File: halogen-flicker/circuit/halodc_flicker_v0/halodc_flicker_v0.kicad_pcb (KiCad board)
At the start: 2 copper layers, 86.1 x 45.6 mm, 21 parts, among them J1 ASP, J2 BATT_LAMP, J4 CHARGER, Q1 IRF540N, SW1 SW_DIP_x02, SW2 SW_Push, U1 ATtiny13A-S, U2 PC817, U3 AMS1117-5.0

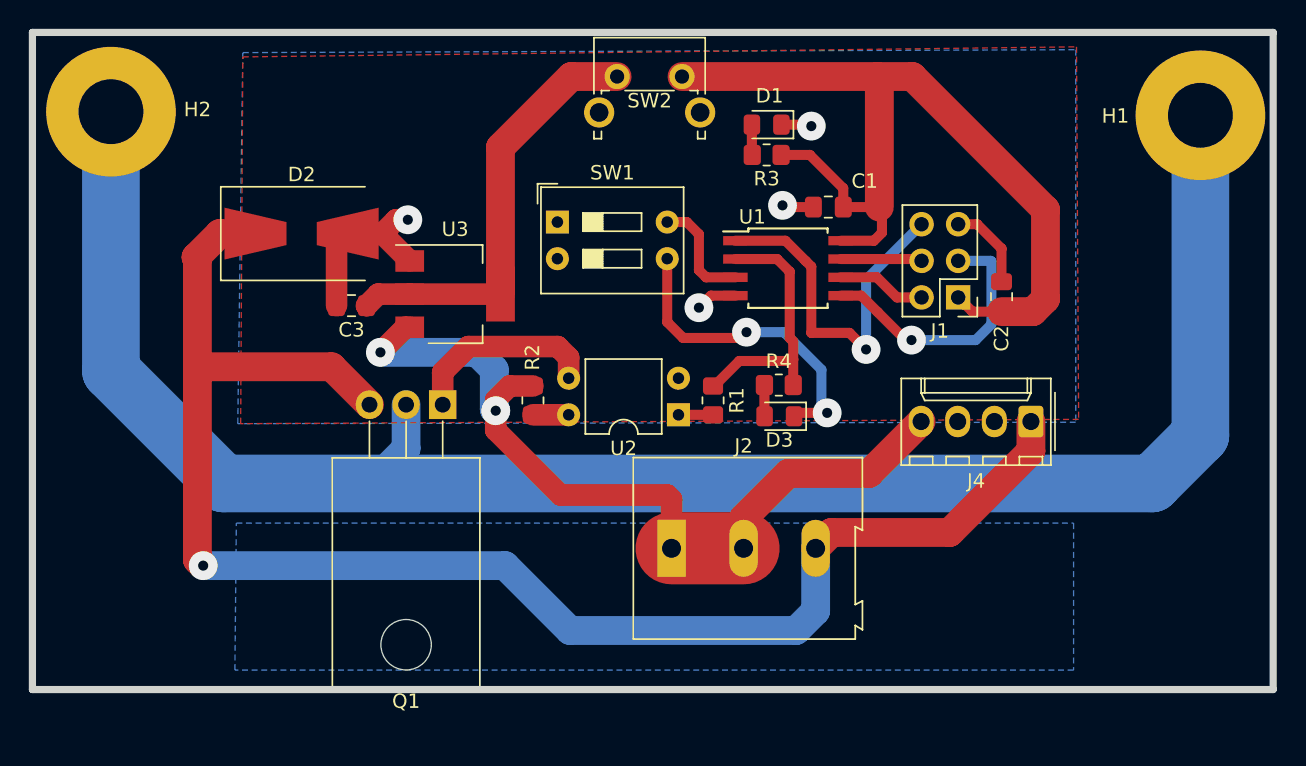
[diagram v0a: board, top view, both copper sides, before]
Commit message: Update PCB FLicker Halogen
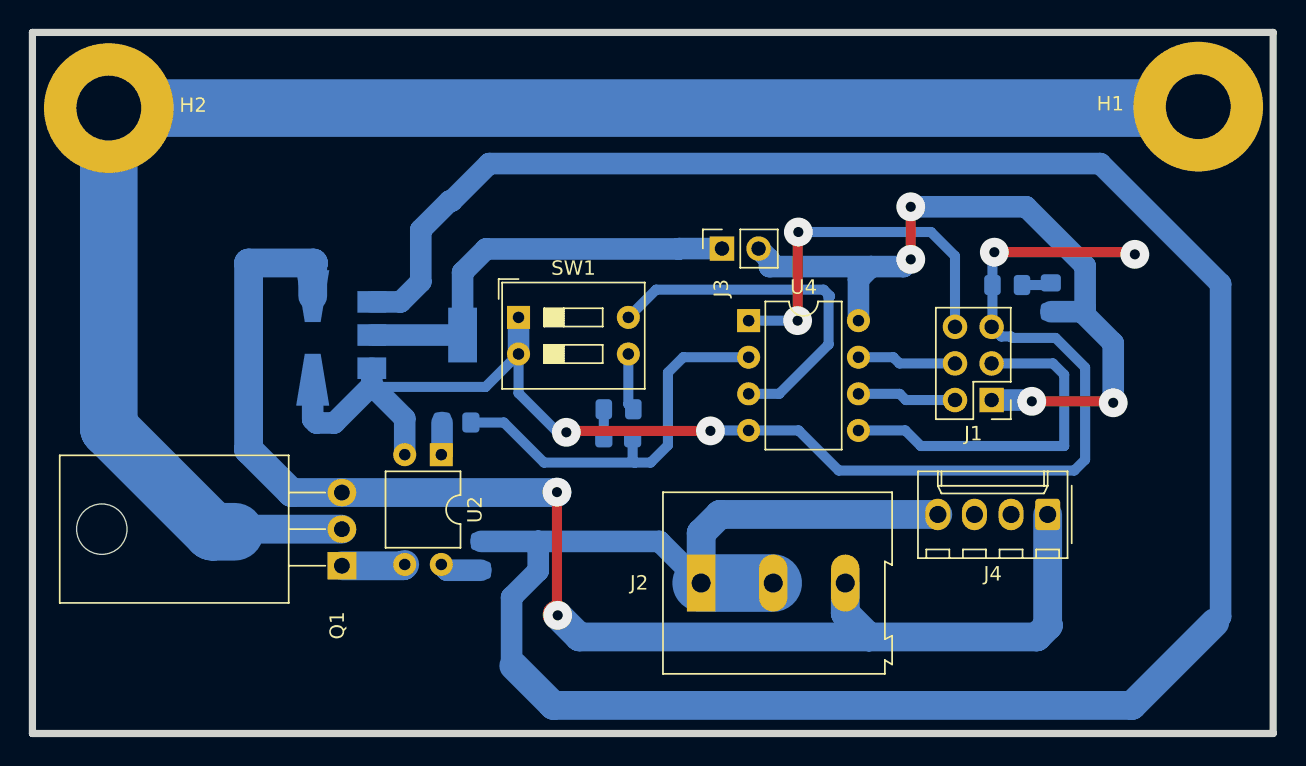
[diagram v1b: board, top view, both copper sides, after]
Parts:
- removed C1, C2, C3: 100nF, Capacitor_SMD:C_0805_2012Metric_Pad1.18x1.45mm_HandSolder
- removed SW2: SW_Push, Button_Switch_THT:SW_Tactile_SPST_Angled_PTS645Vx31-2LFS
- removed U1: ATtiny13A-S, Package_SO:SOIC-8W_5.3x5.3mm_P1.27mm
- added J3: SW_ON, Connector_PinSocket_2.54mm:PinSocket_1x02_P2.54mm_Vertical, F.Cu at (121.2, 54.5)
- added U4: ATtiny13A-P, Package_DIP:DIP-8_W7.62mm, F.Cu at (123.0, 59.5)
- D1, D3, R1, R2, R3, R4, U3: moved to B.Cu
- D2: footprint Diode_SMD:D_SMB-SMC_Universal_Handsoldering -> Diode_SMD:D_SMA-SMB_Universal_Handsoldering; moved to B.Cu
- moved R3 22.1 mm to (144.0, 57.8), turned to 90 degrees
- moved D1 20.1 mm to (140.9, 57.0), turned to 0 degrees
- moved R1 17.9 mm to (102.7, 66.5), turned to 180 degrees
- moved U2 16.7 mm to (101.7, 68.8), turned to -90 degrees
- moved Q1 13.2 mm to (94.8, 76.5), turned to 90 degrees
- moved R4 11.7 mm to (114.0, 67.5)
- moved R2 11.4 mm to (104.4, 75.8)
- moved D3 11.2 mm to (114.0, 65.6)
- moved J1 7.49 mm to (139.9, 65.0)
- moved D2 7.28 mm to (92.8, 60.6), turned to -90 degrees
- moved SW1 7.14 mm to (107.0, 59.2)
- moved J4 6.55 mm to (143.8, 72.9)
- moved U3 3.87 mm to (100.0, 60.5)
- moved J2 3.17 mm to (119.7, 77.7)
- moved H1 0.62 mm to (154.2, 44.6)
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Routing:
- net +12V: track 58.9 -> 195.6 mm, vias 2 -> 0
- net GND: track 25.8 -> 102.5 mm
- net Net-(D3-K): track 22.4 -> 3.98 mm, vias 2 -> 0
- net SEL: track 7.78 -> 25.3 mm
- net +5V: track 65.2 -> 54.7 mm, vias 0 -> 4
- net GNDREF: track 108.5 -> 98.1 mm, vias 1 -> 2
- net CON: track 18.4 -> 28.2 mm
- net Net-(Q1-G): track 13.5 -> 4.40 mm
- net GNDPWR: track 125.6 -> 117.1 mm
- net MOSI: track 18.9 -> 25.0 mm, vias 1 -> 0
- net SCK: track 5.67 -> 6.88 mm
- net NRST: track 25.2 -> 26.0 mm, vias 1 -> 2
- net MISO: track 6.20 -> 6.88 mm
- net Net-(J3-Pin_1): track 29.9 -> 29.3 mm
- added copper zone on B.Cu, net (none)
- removed copper zone on F.Cu, net (none)
- removed copper zone on B.Cu, net GND
- removed copper zone on B.Cu, net GNDREF
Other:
- board size 86.1 x 45.6 mm -> 86.1 x 48.6 mm

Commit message: Update PCB FLicker
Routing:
- added copper zone on F.Cu, net (none)
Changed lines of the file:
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@@
     (fp_line (start 8.89 2.88) (end 8.89 -2.92)
       (stroke (width 0.1) (type solid)) (layer "F.Fab"))
-    (pad "1" thru_hole roundrect (at 0 0 180) (size 1.74 2.19) (drill 1.19) (layers "*.Cu" "*.Mask") (roundrect_rratio 0.143678)
+    (pad "1" thru_hole roundrect (at 0 0 180) (size 1.74 2.19) (drill 1.19) (layers "*.Cu" "*.Mask") (roundrect_rratio 0.1436781609)
       (net 5 "GNDREF") (pinfunction "Pin_1") (pintype "passive"))
     (pad "2" thru_hole oval (at 2.54 0 180) (size 1.74 2.19) (drill 1.19) (layers "*.Cu" "*.Mask")
@@
     (fp_line (start 1 0.625) (end 1 -0.625)
       (stroke (width 0.1) (type solid)) (layer "B.Fab"))
-    (pad "1" smd roundrect (at -1 0 90) (size 1.2 1.4) (layers "B.Cu" "B.Paste" "B.Mask") (roundrect_rratio 0.208333)
+    (pad "1" smd roundrect (at -1 0 90) (size 1.2 1.4) (layers "B.Cu" "B.Paste" "B.Mask") (roundrect_rratio 0.2083333333)
       (net 1 "+5V") (pintype "passive"))
-    (pad "2" smd roundrect (at 1 0 90) (size 1.2 1.4) (layers "B.Cu" "B.Paste" "B.Mask") (roundrect_rratio 0.208333)
+    (pad "2" smd roundrect (at 1 0 90) (size 1.2 1.4) (layers "B.Cu" "B.Paste" "B.Mask") (roundrect_rratio 0.2083333333)
       (net 4 "Net-(D1-A)") (pintype "passive"))
     (model "${KICAD6_3DMODEL_DIR}/Resistor_SMD.3dshapes/R_0805_2012Metric.wrl"
@@
     (fp_line (start 1 0.625) (end 1 -0.625)
       (stroke (width 0.1) (type solid)) (layer "B.Fab"))
-    (pad "1" smd roundrect (at -1 0) (size 1.2 1.4) (layers "B.Cu" "B.Paste" "B.Mask") (roundrect_rratio 0.208333)
+    (pad "1" smd roundrect (at -1 0) (size 1.2 1.4) (layers "B.Cu" "B.Paste" "B.Mask") (roundrect_rratio 0.2083333333)
       (net 7 "Net-(D3-A)") (pintype "passive"))
-    (pad "2" smd roundrect (at 1 0) (size 1.2 1.4) (layers "B.Cu" "B.Paste" "B.Mask") (roundrect_rratio 0.208333)
+    (pad "2" smd roundrect (at 1 0) (size 1.2 1.4) (layers "B.Cu" "B.Paste" "B.Mask") (roundrect_rratio 0.2083333333)
       (net 17 "CON") (pintype "passive"))
     (model "${KICAD6_3DMODEL_DIR}/Resistor_SMD.3dshapes/R_0805_2012Metric.wrl"
@@
     (fp_line (start 1 0.6) (end -0.7 0.6)
       (stroke (width 0.1) (type solid)) (layer "B.Fab"))
-    (pad "1" smd roundrect (at -1.025 0) (size 1.15 1.4) (layers "B.Cu" "B.Paste" "B.Mask") (roundrect_rratio 0.217391)
+    (pad "1" smd roundrect (at -1.025 0) (size 1.15 1.4) (layers "B.Cu" "B.Paste" "B.Mask") (roundrect_rratio 0.2173913043)
       (net 2 "GND") (pinfunction "K") (pintype "passive"))
-    (pad "2" smd roundrect (at 1.025 0) (size 1.15 1.4) (layers "B.Cu" "B.Paste" "B.Mask") (roundrect_rratio 0.217391)
+    (pad "2" smd roundrect (at 1.025 0) (size 1.15 1.4) (layers "B.Cu" "B.Paste" "B.Mask") (roundrect_rratio 0.2173913043)
       (net 4 "Net-(D1-A)") (pinfunction "A") (pintype "passive"))
     (model "${KICAD6_3DMODEL_DIR}/LED_SMD.3dshapes/LED_0805_2012Metric.wrl"
@@
     (fp_line (start 1 0.6) (end -0.7 0.6)
       (stroke (width 0.1) (type solid)) (layer "B.Fab"))
-    (pad "1" smd roundrect (at -1.025 0 180) (size 1.15 1.4) (layers "B.Cu" "B.Paste" "B.Mask") (roundrect_rratio 0.217391)
+    (pad "1" smd roundrect (at -1.025 0 180) (size 1.15 1.4) (layers "B.Cu" "B.Paste" "B.Mask") (roundrect_rratio 0.2173913043)
       (net 6 "Net-(D3-K)") (pinfunction "K") (pintype "passive"))
-    (pad "2" smd roundrect (at 1.025 0 180) (size 1.15 1.4) (layers "B.Cu" "B.Paste" "B.Mask") (roundrect_rratio 0.217391)
+    (pad "2" smd roundrect (at 1.025 0 180) (size 1.15 1.4) (layers "B.Cu" "B.Paste" "B.Mask") (roundrect_rratio 0.2173913043)
       (net 7 "Net-(D3-A)") (pinfunction "A") (pintype "passive"))
     (model "${KICAD6_3DMODEL_DIR}/LED_SMD.3dshapes/LED_0805_2012Metric.wrl"
@@
     (fp_line (start 1 0.625) (end 1 -0.625)
       (stroke (width 0.1) (type solid)) (layer "B.Fab"))
-    (pad "1" smd roundrect (at -1 0 180) (size 1.2 1.4) (layers "B.Cu" "B.Paste" "B.Mask") (roundrect_rratio 0.208333)
+    (pad "1" smd roundrect (at -1 0 180) (size 1.2 1.4) (layers "B.Cu" "B.Paste" "B.Mask") (roundrect_rratio 0.2083333333)
       (net 17 "CON") (pintype "passive"))
-    (pad "2" smd roundrect (at 1 0 180) (size 1.2 1.4) (layers "B.Cu" "B.Paste" "B.Mask") (roundrect_rratio 0.208333)
+    (pad "2" smd roundrect (at 1 0 180) (size 1.2 1.4) (layers "B.Cu" "B.Paste" "B.Mask") (roundrect_rratio 0.2083333333)
       (net 18 "Net-(R1-Pad2)") (pintype "passive"))
     (model "${KICAD6_3DMODEL_DIR}/Resistor_SMD.3dshapes/R_0805_2012Metric.wrl"
@@
     (fp_line (start 1 0.625) (end 1 -0.625)
       (stroke (width 0.1) (type solid)) (layer "B.Fab"))
-    (pad "1" smd roundrect (at -1 0 90) (size 1.2 1.4) (layers "B.Cu" "B.Paste" "B.Mask") (roundrect_rratio 0.208333)
+    (pad "1" smd roundrect (at -1 0 90) (size 1.2 1.4) (layers "B.Cu" "B.Paste" "B.Mask") (roundrect_rratio 0.2083333333)
       (net 19 "Net-(R2-Pad1)") (pintype "passive"))
-    (pad "2" smd roundrect (at 1 0 90) (size 1.2 1.4) (layers "B.Cu" "B.Paste" "B.Mask") (roundrect_rratio 0.208333)
+    (pad "2" smd roundrect (at 1 0 90) (size 1.2 1.4) (layers "B.Cu" "B.Paste" "B.Mask") (roundrect_rratio 0.2083333333)
       (net 13 "+12V") (pintype "passive"))
     (model "${KICAD6_3DMODEL_DIR}/Resistor_SMD.3dshapes/R_0805_2012Metric.wrl"
@@
   (segment (start 125.12 64.53) (end 128.55 61.1) (width 0.7) (layer "B.Cu") (net 20))
   (segment (start 123 64.53) (end 125.12 64.53) (width 0.7) (layer "B.Cu") (net 20))
+  (zone (net 0) (net_name "") (layer "F.Cu") (hatch edge 0.5)
+    (priority 1)
+    (connect_pads (clearance 1))
+    (min_thickness 0.25) (filled_areas_thickness no)
+    (fill yes (thermal_gap 0.5) (thermal_bridge_width 0.5) (island_removal_mode 1) (island_area_min 10))
+    (polygon
+      (pts
+        (xy 73.3 39.35)
+        (xy 159.45 39.55)
+        (xy 159.5 88.1)
+        (xy 73.4 88.05)
+      )
+    )
+  )
   (zone (net 0) (net_name "") (layer "B.Cu") (hatch edge 0.5)
     (connect_pads (clearance 1.5))

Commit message: Halogen and ATTiny is hard
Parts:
- R1: value 100 -> 10K
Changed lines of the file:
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@@
         (effects (font (size 1 1) (thickness 0.15)) (justify mirror))
     )
-    (fp_text value "100" (at 0 -1.65) (layer "B.Fab")
+    (fp_text value "10K" (at 0 -1.65) (layer "B.Fab")
         (effects (font (size 1 1) (thickness 0.15)) (justify mirror))
     )
